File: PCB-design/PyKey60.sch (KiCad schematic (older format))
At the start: 278 parts, among them J1 USB_C_Receptacle_USB2.0, J2 Conn_01x03, J3 Conn_01x04, J4 Conn_01x06, SW1 SW_SPST, SW2 SW_SPDT, U1 CherryMX_LTST-A683CEGBW, U10 CherryMX_LTST-A683CEGBW, U11 CherryMX_LTST-A683CEGBW, U12 CherryMX_LTST-A683CEGBW, U13 CherryMX_LTST-A683CEGBW, U14 CherryMX_LTST-A683CEGBW, U15 CherryMX_LTST-A683CEGBW, U16 CherryMX_LTST-A683CEGBW, U17 CherryMX_LTST-A683CEGBW, U18 CherryMX_LTST-A683CEGBW, U19 CherryMX_LTST-A683CEGBW, U2 CherryMX_LTST-A683CEGBW, U20 CherryMX_LTST-A683CEGBW, U21 CherryMX_LTST-A683CEGBW, U22 CherryMX_LTST-A683CEGBW, U23 CherryMX_LTST-A683CEGBW, U24 CherryMX_LTST-A683CEGBW, U25 CherryMX_LTST-A683CEGBW, U26 CherryMX_LTST-A683CEGBW, U27 CherryMX_LTST-A683CEGBW, U28 CherryMX_LTST-A683CEGBW, U29 CherryMX_LTST-A683CEGBW, U3 CherryMX_LTST-A683CEGBW, U30 CherryMX_LTST-A683CEGBW, U31 CherryMX_LTST-A683CEGBW, U32 CherryMX_LTST-A683CEGBW, U33 CherryMX_LTST-A683CEGBW, U34 CherryMX_LTST-A683CEGBW, U35 CherryMX_LTST-A683CEGBW, U36 CherryMX_LTST-A683CEGBW, U37 CherryMX_LTST-A683CEGBW, U38 CherryMX_LTST-A683CEGBW, U39 CherryMX_LTST-A683CEGBW, U4 CherryMX_LTST-A683CEGBW, U40 CherryMX_LTST-A683CEGBW, U41 CherryMX_LTST-A683CEGBW, U42 CherryMX_LTST-A683CEGBW, U43 CherryMX_LTST-A683CEGBW, U44 CherryMX_LTST-A683CEGBW, U45 CherryMX_LTST-A683CEGBW, U46 CherryMX_LTST-A683CEGBW, U47 CherryMX_LTST-A683CEGBW, U48 CherryMX_LTST-A683CEGBW, U49 CherryMX_LTST-A683CEGBW, U5 CherryMX_LTST-A683CEGBW, U50 CherryMX_LTST-A683CEGBW, U51 CherryMX_LTST-A683CEGBW, U52 CherryMX_LTST-A683CEGBW, U53 CherryMX_LTST-A683CEGBW, U54 CherryMX_LTST-A683CEGBW, U55 CherryMX_LTST-A683CEGBW, U56 CherryMX_LTST-A683CEGBW, U57 CherryMX_LTST-A683CEGBW, U58 CherryMX_LTST-A683CEGBW, U59 CherryMX_LTST-A683CEGBW, U6 CherryMX_LTST-A683CEGBW, U60 CherryMX_LTST-A683CEGBW, U61 CherryMX_LTST-A683CEGBW, U62 RP2040, U63 USBLC6-2SC6, U64 W25Q128JVS, U65 AMS1117-3.3, U66 CherryMX_LTST-A683CEGBW, U67 CherryMX_LTST-A683CEGBW, U68 CherryMX_LTST-A683CEGBW, U69 CherryMX_LTST-A683CEGBW, U7 CherryMX_LTST-A683CEGBW, U70 CherryMX_LTST-A683CEGBW, U71 CherryMX_LTST-A683CEGBW, U72 CherryMX_LTST-A683CEGBW, U73 CherryMX_LTST-A683CEGBW, U74 CherryMX_LTST-A683CEGBW, U75 CherryMX_LTST-A683CEGBW, U76 CherryMX_LTST-A683CEGBW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

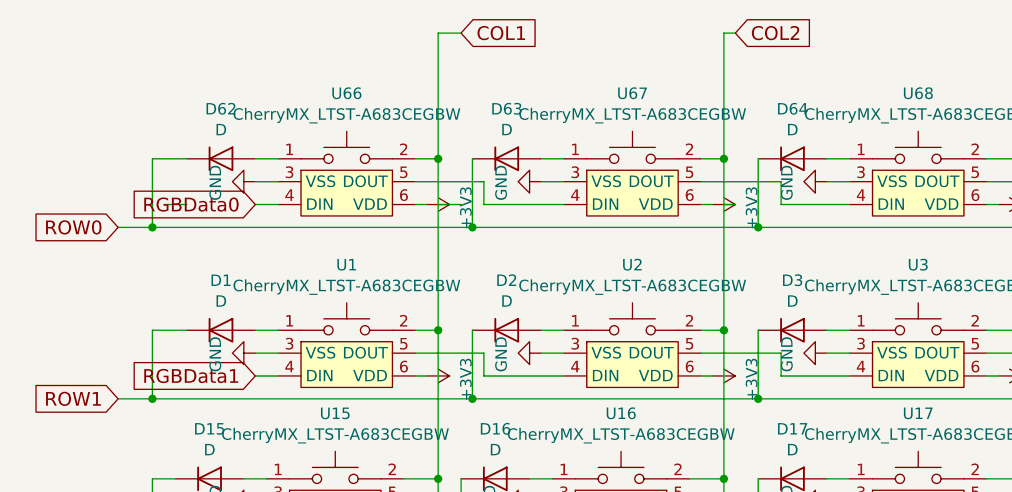
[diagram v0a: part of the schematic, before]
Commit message: adding more connections
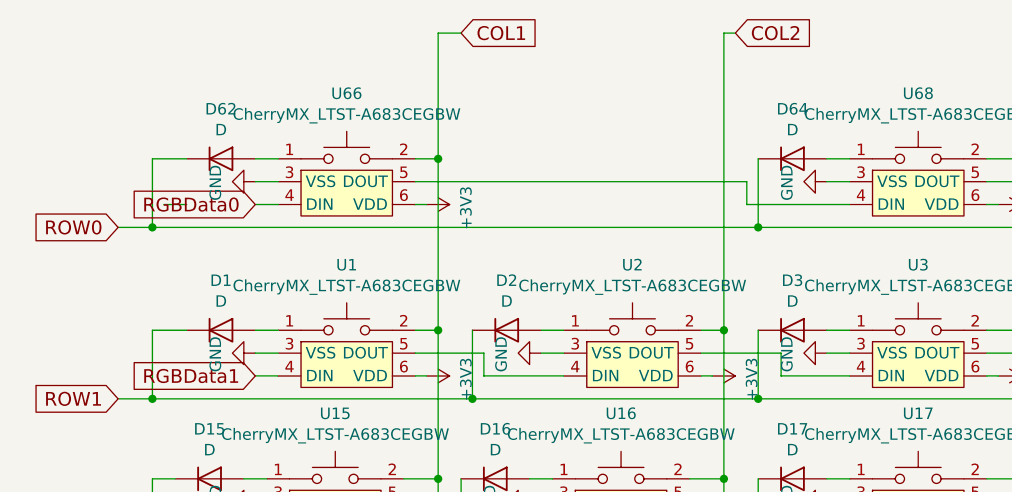
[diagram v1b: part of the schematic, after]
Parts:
- removed D63: D, Diode_SMD:D_SOD-123, symbol Device:D
- removed U67: CherryMX_LTST-A683CEGBW, CherryMX_PCB_KailhSocket_LTST-A683CEGBW-Rotated-HS:CherryMX_1.00u_PCB_KailhSocket_LTST-A683CEGBW-Rotated-HS, symbol CherryMX:CherryMX_LTST-A683CEGBW
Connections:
- wire segments 1307 -> 1295
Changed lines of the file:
@@
 	4200 1650 4300 1650
 Wire Wire Line
-	3800 1100 3750 1100
-Wire Wire Line
 	3750 4550 3600 4550
 Wire Wire Line
@@
 	2500 1650 2500 2300
 Wire Wire Line
-	2500 1100 2600 1100
-Wire Wire Line
 	2400 1650 2500 1650
 Wire Wire Line
@@
 	7700 1100 7600 1100
 $Comp
-L CherryMX:CherryMX_LTST-A683CEGBW U67
-U 1 1 622342B5
-P 3350 1000
-F 0 "U67" H 3350 1385 50  0000 C CNN
-F 1 "CherryMX_LTST-A683CEGBW" H 3350 1294 50  0000 C CNN
-F 2 "CherryMX_PCB_KailhSocket_LTST-A683CEGBW-Rotated-HS:CherryMX_1.00u_PCB_KailhSocket_LTST-A683CEGBW-Rotated-HS" H 3350 900 50  0001 C CNN
-F 3 "" H 3350 900 50  0001 C CNN
-	1    3350 1000
-	1    0    0    -1
-$EndComp
-$Comp
-L Device:D D63
-U 1 1 622342BB
-P 2800 900
-F 0 "D63" H 2800 1117 50  0000 C CNN
-F 1 "D" H 2800 1026 50  0000 C CNN
-F 2 "Diode_SMD:D_SOD-123" H 2800 900 50  0001 C CNN
-F 3 "~" H 2800 900 50  0001 C CNN
-	1    2800 900
-	1    0    0    -1
-$EndComp
-$Comp
 L CherryMX:CherryMX_LTST-A683CEGBW U68
 U 1 1 622342C1
@@
 COL2
 Wire Wire Line
-	2650 1200 2650 900
-Wire Wire Line
-	2650 1200 3900 1200
-Wire Wire Line
 	3900 1200 3900 900
 Wire Wire Line
-	2950 900  3050 900
-Wire Wire Line
 	4200 900  4300 900
 Wire Wire Line
 	3800 350  3750 350
 Wire Wire Line
-	3750 350  3750 900
-Wire Wire Line
-	3650 900  3750 900
-Connection ~ 3750 900
-Wire Wire Line
 	3900 1200 5150 1200
 Wire Wire Line
 	5150 1200 5150 900
-Connection ~ 3900 1200
 Wire Wire Line
 	5150 1200 6450 1200
@@
 	16700 1150 17000 1150
 Wire Wire Line
-	2700 1000 2700 1100
-Wire Wire Line
-	2700 1100 3050 1100
-Wire Wire Line
-	3650 1000 4000 1000
-Wire Wire Line
-	4000 1000 4000 1100
-Wire Wire Line
-	4000 1100 4300 1100
-Wire Wire Line
 	4900 1000 5200 1000
 Wire Wire Line
@@
 	6500 1100 6850 1100
 $Comp
-L power:GND #PWR0239
-U 1 1 622343F7
-P 2950 1000
-F 0 "#PWR0239" H 2950 750 50  0001 C CNN
-F 1 "GND" H 2955 827 50  0000 C CNN
-F 2 "" H 2950 1000 50  0001 C CNN
-F 3 "" H 2950 1000 50  0001 C CNN
-	1    2950 1000
-	0    1    1    0
-$EndComp
-$Comp
 L power:GND #PWR0240
 U 1 1 622343FD
@@
 $EndComp
 Wire Wire Line
-	2950 1000 3050 1000
-Wire Wire Line
 	4200 1000 4300 1000
 Wire Wire Line
@@
 	14450 1050 14350 1050
 $Comp
-L power:+3V3 #PWR0252
-U 1 1 62234452
-P 3700 1100
-F 0 "#PWR0252" H 3700 950 50  0001 C CNN
-F 1 "+3V3" H 3715 1273 50  0000 C CNN
-F 2 "" H 3700 1100 50  0001 C CNN
-F 3 "" H 3700 1100 50  0001 C CNN
-	1    3700 1100
-	0    1    1    0
-$EndComp
-$Comp
 L power:+3V3 #PWR0253
 U 1 1 62234458
@@
 	4950 1100 4900 1100
 Wire Wire Line
-	3700 1100 3650 1100
-Wire Wire Line
 	7450 1100 7500 1100
 Wire Wire Line
@@
 	0    1    1    0
 $EndComp
-Connection ~ 2650 1200
 Wire Wire Line
 	2450 1100 2400 1100
@@
 $EndComp
 Wire Wire Line
-	2400 1000 2700 1000
-Wire Wire Line
 	1700 1100 1800 1100
 Text GLabel 1700 1100 0    60   Input ~ 0
 RGBData0
 Connection ~ 1250 1200
-Wire Wire Line
-	1250 1200 2650 1200
 Connection ~ 2500 900
 Wire Wire Line
@@
 	7700 350  7600 350
 Wire Wire Line
-	3750 900  3750 1650
-Wire Wire Line
 	5050 900  5050 1650
 Wire Wire Line
@@
 Wire Wire Line
 	11200 9650 11350 9650
+Wire Wire Line
+	3750 350  3750 1650
+Wire Wire Line
+	3850 1000 3850 1100
+Wire Wire Line
+	2400 1000 3850 1000
+Wire Wire Line
+	3850 1100 4300 1100
+Connection ~ 3900 1200
+Wire Wire Line
+	1250 1200 3900 1200
 $EndSCHEMATC
